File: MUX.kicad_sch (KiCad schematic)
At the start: 18 parts, among them U2 74HC4051, U32 74HC4051, U38 74HC4051, U45 74HC4051, U51 74HC4051, U56 74HC4051, U62 74HC4051, U69 74HC4051, U74 74HC4051

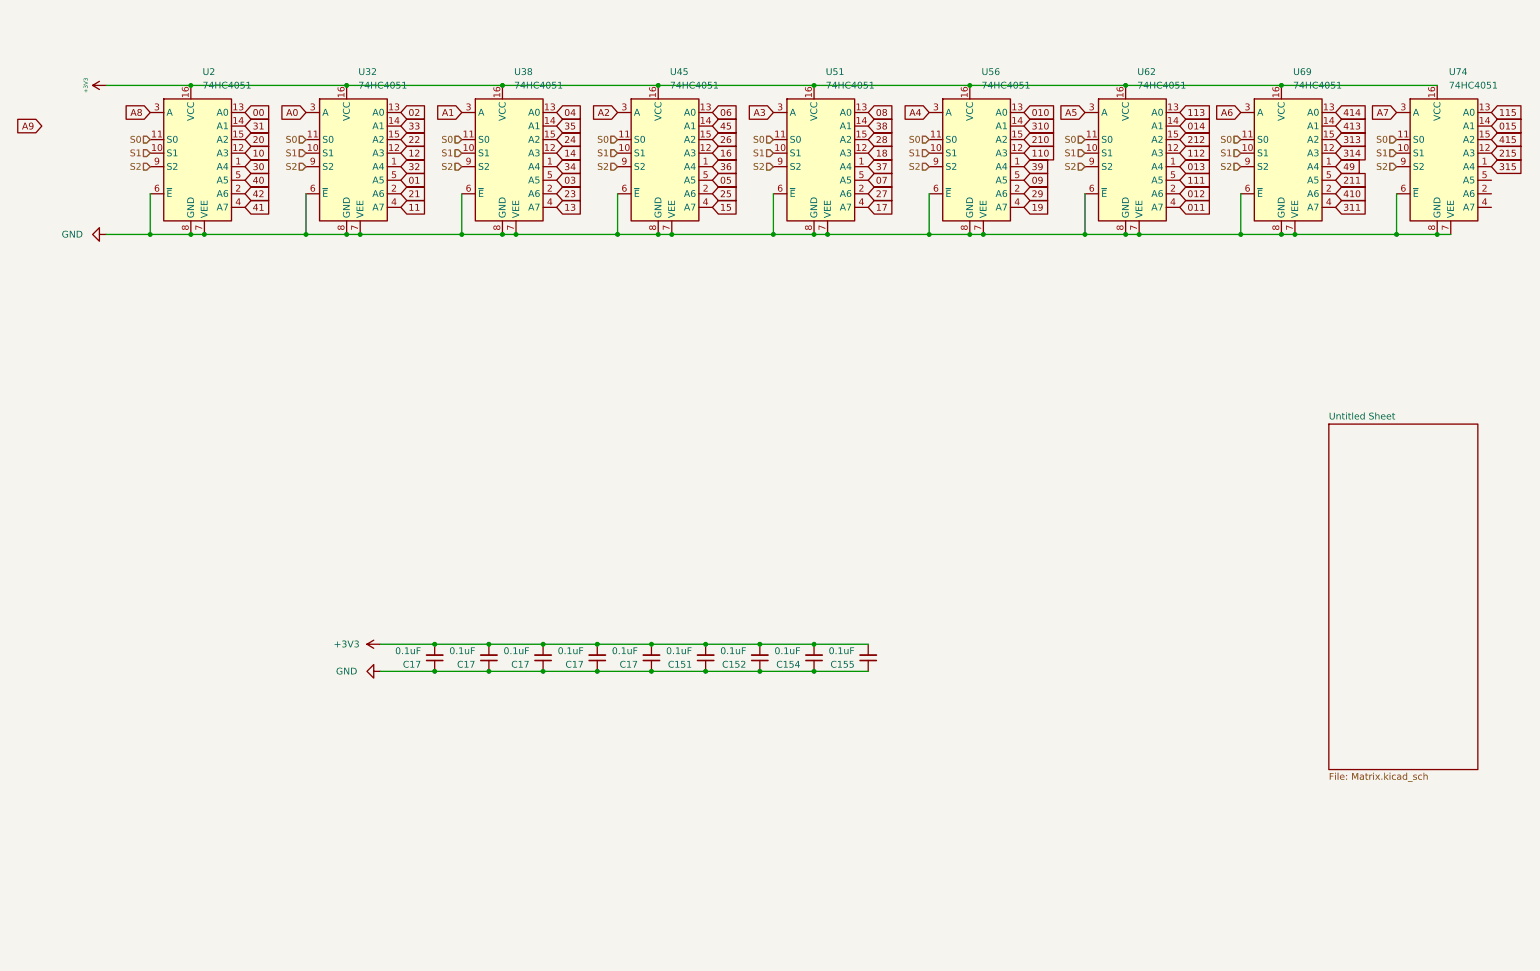
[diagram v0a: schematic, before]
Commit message: a
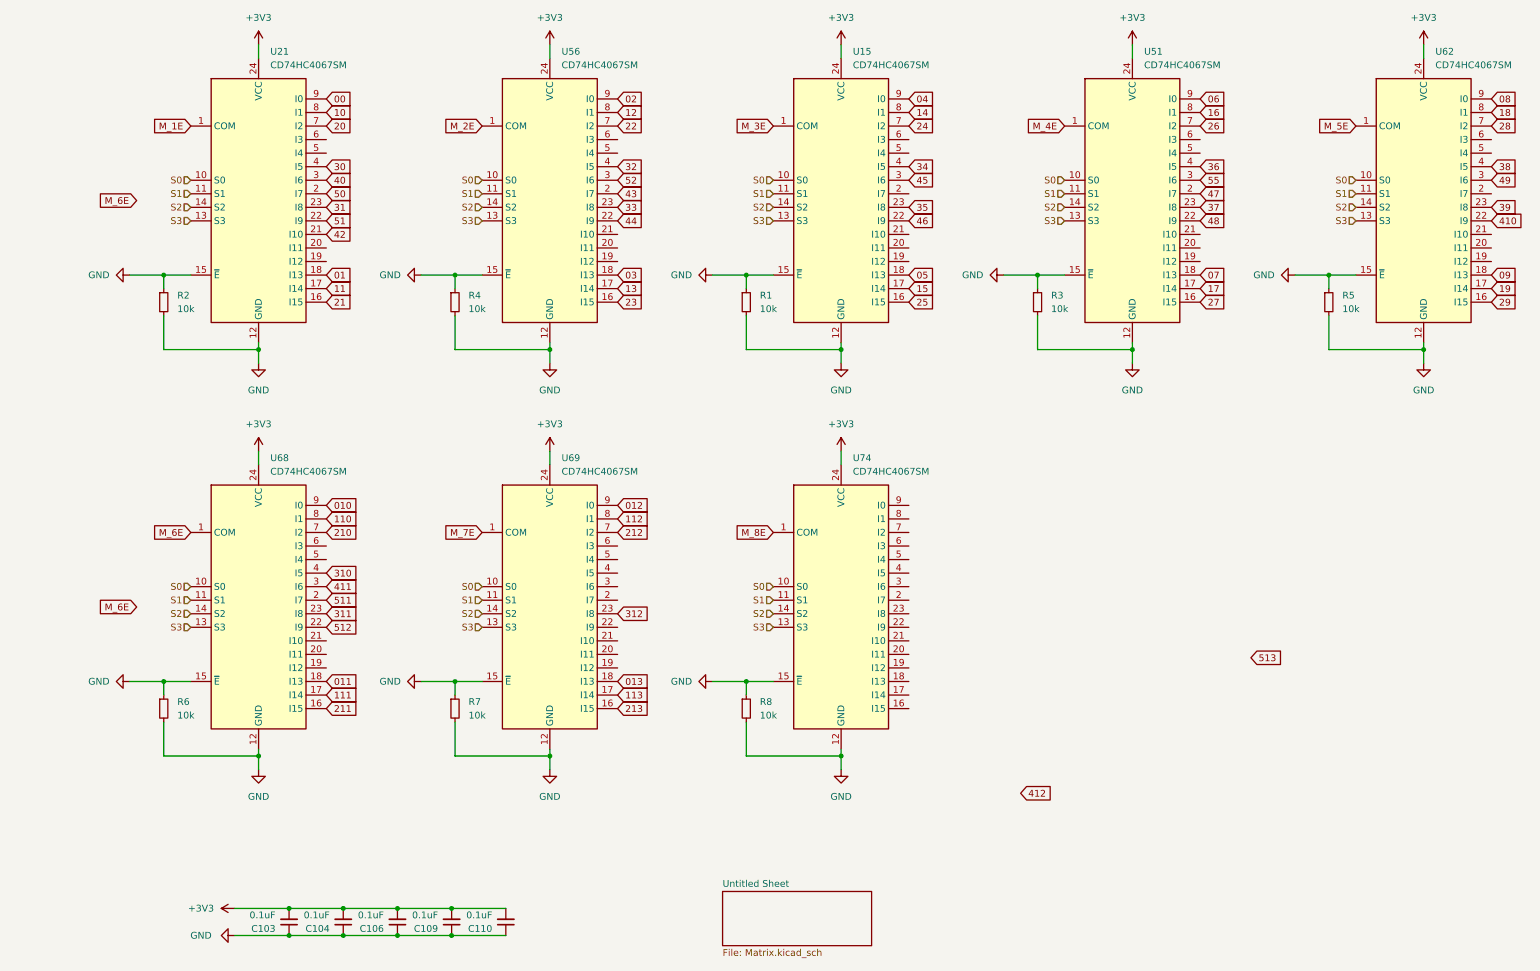
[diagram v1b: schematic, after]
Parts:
- removed C151, C152, C154, C155, C17 (x5): 0.1uF, Common_Footprint:C_0402, symbol Device:C_Small
- removed U2, U32, U38, U45, U51, U56, U62, U69, U74: 74HC4051, Package_SO:SSOP-16_4.4x5.2mm_P0.65mm, symbol 74xx:74HC4051
- added C103, C104, C106, C109, C110: 0.1uF, sanproject-keyboard-part-v6:C_0402, symbol Device:C_Small
- added R1, R2, R3, R4, R5, R6, R7, R8: 10k, sanproject-keyboard-part:R_0402, symbol Device:R_Small
- added U15, U21, U51, U56, U62, U68, U69, U74: CD74HC4067SM, Package_SO:TSSOP-24_4.4x7.8mm_P0.65mm, symbol 74xx:CD74HC4067SM
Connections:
- net +3V3: now also C103.2, C104.2, C106.2, C109.2, C110.2, U15.24 (VCC), U21.24 (VCC), U51.24 (VCC), U56.24 (VCC), U62.24 (VCC), U68.24 (VCC), U69.24 (VCC), U74.24 (VCC)
- net 00: now also U21.9 (I0)
- net 01: now also U21.18 (I13)
- net 010: now also U68.9 (I0)
- net 011: now also U68.18 (I13)
- net 012: now also U69.9 (I0)
- net 013: now also U69.18 (I13)
- net 02: now also U56.9 (I0)
- net 03: now also U56.18 (I13)
- net 04: now also U15.9 (I0)
- net 05: now also U15.18 (I13)
- net 06: now also U51.9 (I0)
- net 07: now also U51.18 (I13)
- net 08: now also U62.9 (I0)
- net 09: now also U62.18 (I13)
- net 10: now also U21.8 (I1)
- net 11: now also U21.17 (I14)
- net 110: now also U68.8 (I1)
- net 111: now also U68.17 (I14)
- net 112: now also U69.8 (I1)
- net 113: now also U69.17 (I14)
- net 12: now also U56.8 (I1)
- net 13: now also U56.17 (I14)
- net 14: now also U15.8 (I1)
- net 15: now also U15.17 (I14)
- net 16: now also U51.8 (I1)
- net 17: now also U51.17 (I14)
- net 18: now also U62.8 (I1)
- net 19: now also U62.17 (I14)
- net 20: now also U21.7 (I2)
- net 21: now also U21.16 (I15)
- net 210: now also U68.7 (I2)
- net 211: now also U68.16 (I15)
- net 212: now also U69.7 (I2)
- net 22: now also U56.7 (I2)
- net 23: now also U56.16 (I15)
- net 24: now also U15.7 (I2)
- net 25: now also U15.16 (I15)
- net 26: now also U51.7 (I2)
- net 27: now also U51.16 (I15)
- net 28: now also U62.7 (I2)
- net 29: now also U62.16 (I15)
- net 30: now also U21.4 (I5)
- net 31: now also U21.23 (I8)
- net 310: now also U68.4 (I5)
- net 311: now also U68.23 (I8)
- net 32: now also U56.4 (I5)
- net 33: now also U56.23 (I8)
- net 34: now also U15.4 (I5)
- net 35: now also U15.23 (I8)
- net 36: now also U51.4 (I5)
- net 37: now also U51.23 (I8)
- net 38: now also U62.4 (I5)
- net 39: now also U62.23 (I8)
- net 40: now also U21.3 (I6)
- net 410: now also U62.22 (I9)
- net 42: now also U21.21 (I10)
- net 45: now also U15.3 (I6)
- net 49: now also U62.3 (I6)
- net GND: now also C103.1, C104.1, C106.1, C109.1, C110.1, R1.1, R1.2, R2.1, R2.2, R3.1, R3.2, R4.1, R4.2, R5.1, R5.2, R6.1, R6.2, R7.1, R7.2, R8.1, R8.2, U15.12 (GND), U15.15 (~{E}), U21.12 (GND), U21.15 (~{E}), U51.12 (GND), U51.15 (~{E}), U56.12 (GND), U56.15 (~{E}), U62.12 (GND), U62.15 (~{E}), U68.12 (GND), U68.15 (~{E}), U69.12 (GND), U69.15 (~{E}), U74.12 (GND), U74.15 (~{E})
- net S0: now also U15.10 (S0), U21.10 (S0), U51.10 (S0), U56.10 (S0), U62.10 (S0), U68.10 (S0), U69.10 (S0), U74.10 (S0)
- net S1: now also U15.11 (S1), U21.11 (S1), U51.11 (S1), U56.11 (S1), U62.11 (S1), U68.11 (S1), U69.11 (S1), U74.11 (S1)
- net S2: now also U15.14 (S2), U21.14 (S2), U51.14 (S2), U56.14 (S2), U62.14 (S2), U68.14 (S2), U69.14 (S2), U74.14 (S2)
- new net 213: U69.16 (I15)
- new net 312: U69.23 (I8)
- new net 411: U68.3 (I6)
- new net 43: U56.2 (I7)
- new net 44: U56.22 (I9)
- new net 46: U15.22 (I9)
- new net 47: U51.2 (I7)
- new net 48: U51.22 (I9)
- new net 50: U21.2 (I7)
- new net 51: U21.22 (I9)
- new net 511: U68.2 (I7)
- new net 512: U68.22 (I9)
- new net 52: U56.3 (I6)
- new net 55: U51.3 (I6)
- new net M_1E: U21.1 (COM)
- new net M_2E: U56.1 (COM)
- new net M_3E: U15.1 (COM)
- new net M_4E: U51.1 (COM)
- new net M_5E: U62.1 (COM)
- new net M_6E: U68.1 (COM)
- new net M_7E: U69.1 (COM)
- new net M_8E: U74.1 (COM)
- new net S3: U15.13 (S3), U21.13 (S3), U51.13 (S3), U56.13 (S3), U62.13 (S3), U68.13 (S3), U69.13 (S3), U74.13 (S3)
